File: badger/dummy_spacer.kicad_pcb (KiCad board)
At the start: 2 copper layers, 200 x 200 mm, 12 parts

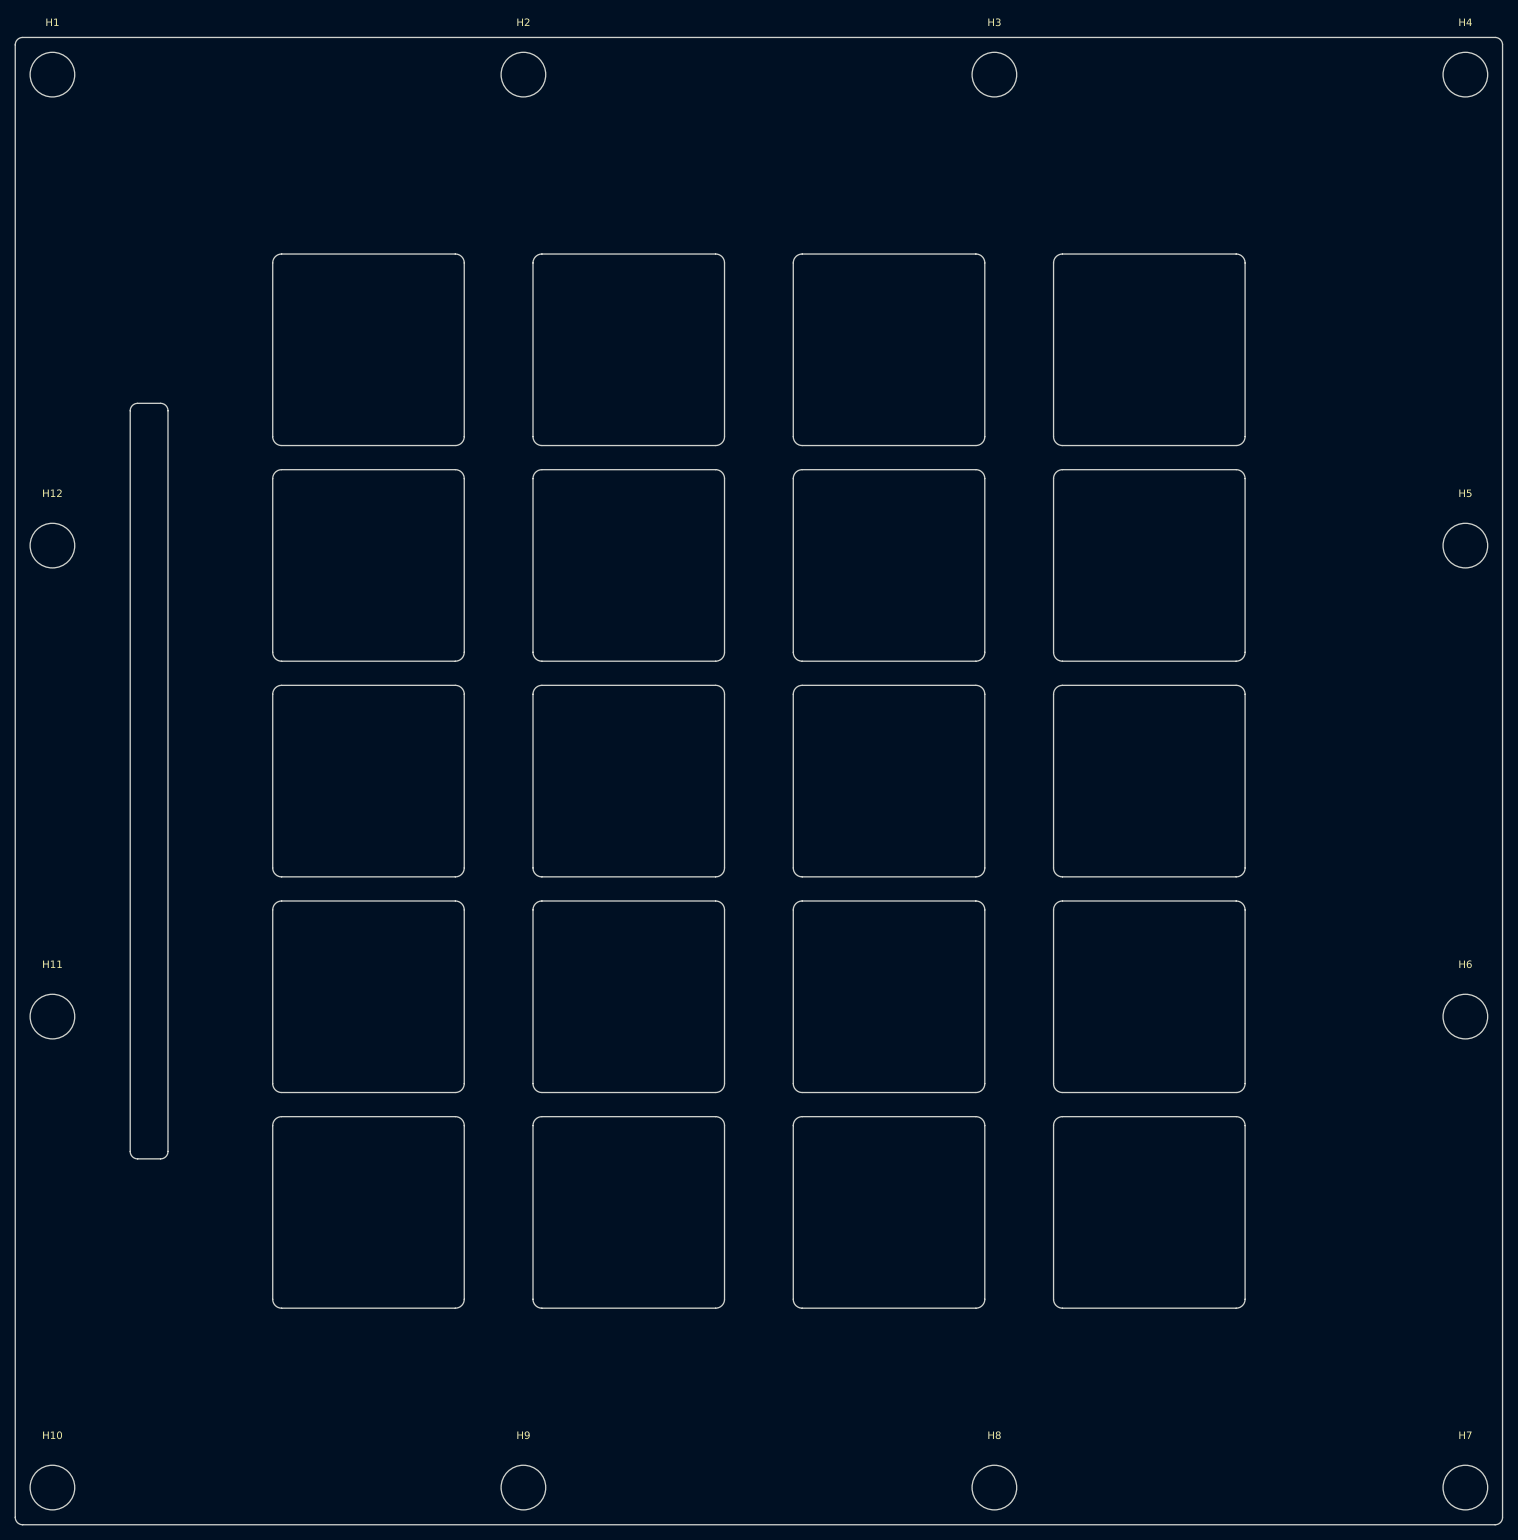
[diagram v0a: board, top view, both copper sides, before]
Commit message: badger upgrades
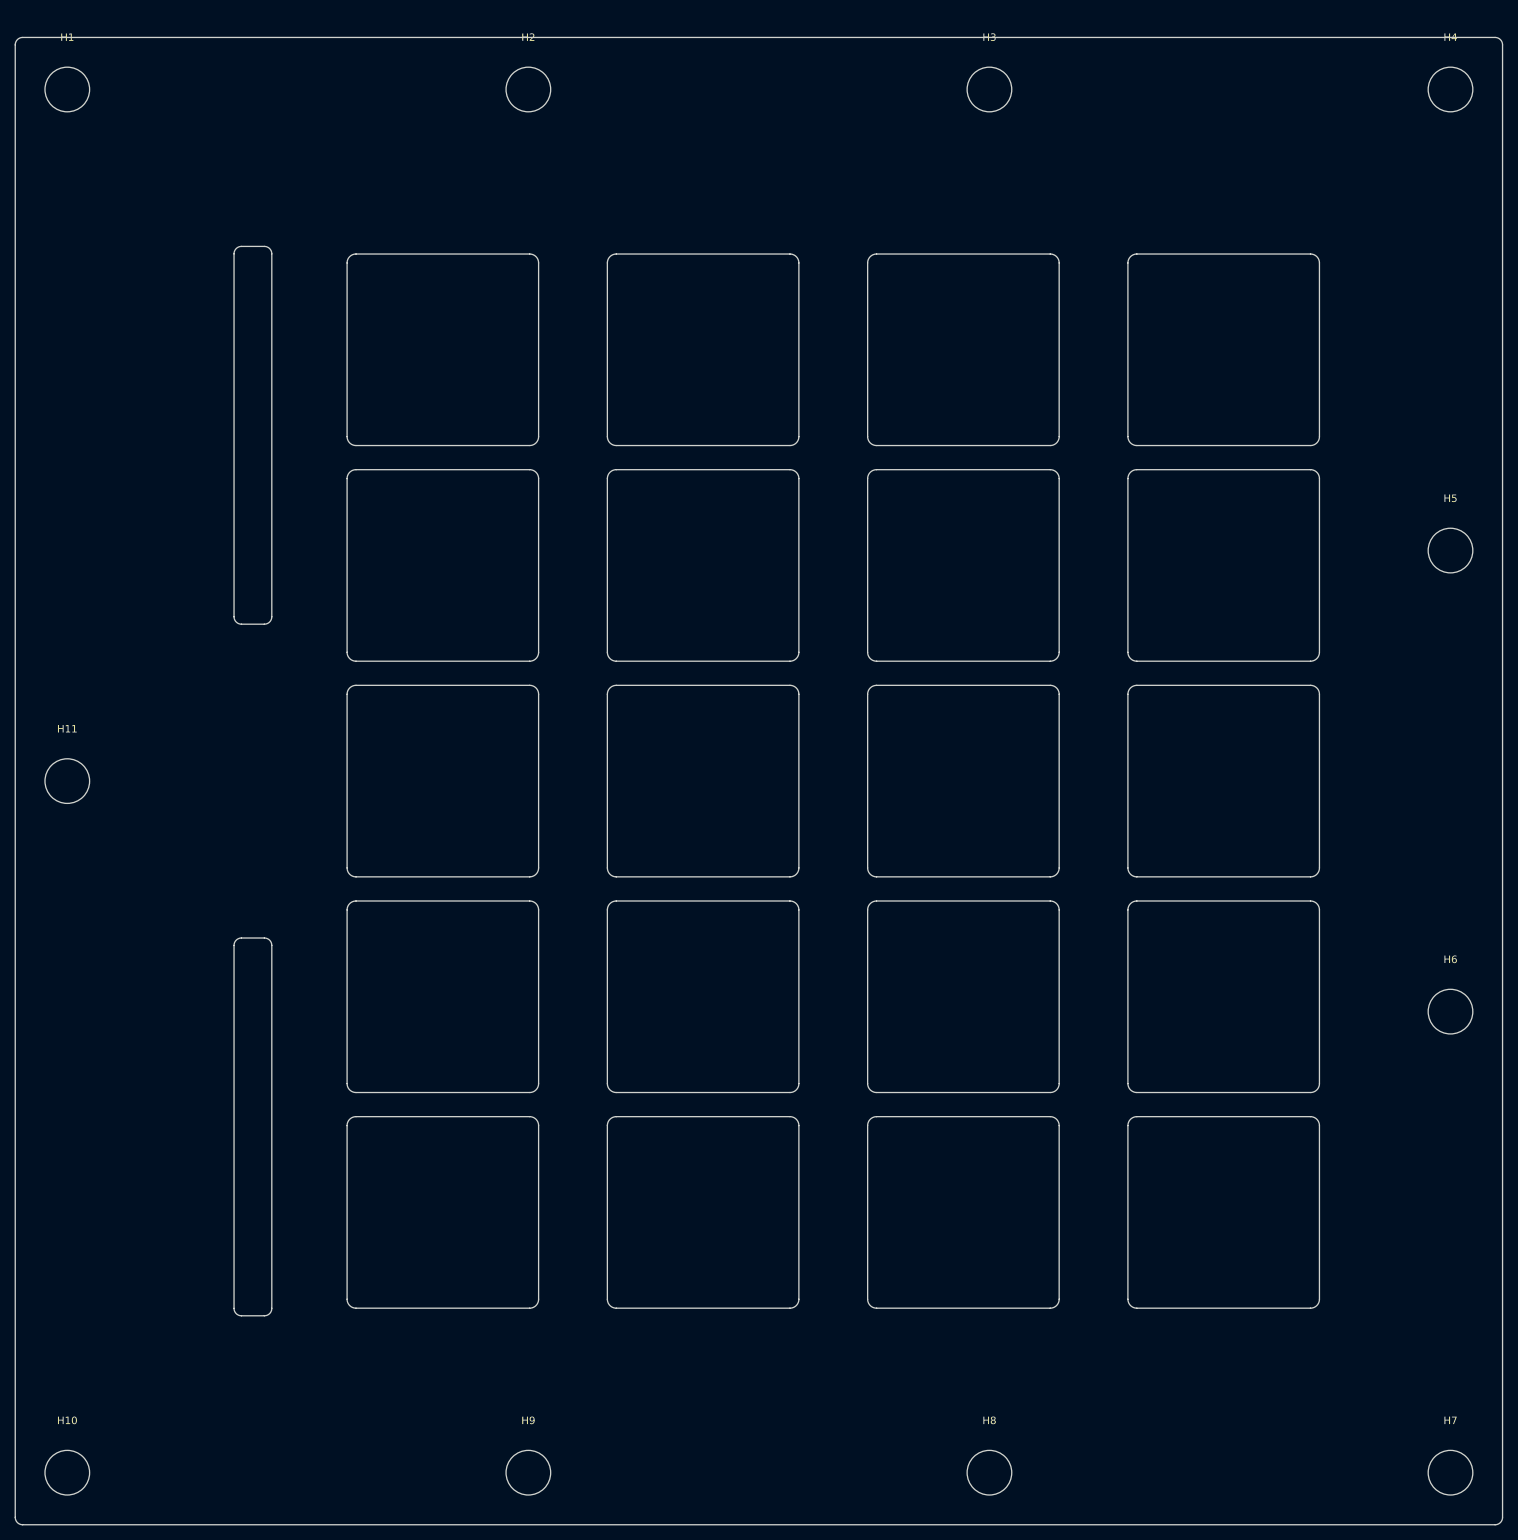
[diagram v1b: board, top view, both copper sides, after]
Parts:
- removed H12: MountingHole, MountingHole:MountingHole_6mm
- moved H11 31.7 mm to (-93.0, 0.00)
- moved H1 2.83 mm to (-93.0, -93.0)
- moved H10 2.83 mm to (-93.0, 93.0)
- moved H4 2.83 mm to (93.0, -93.0)
- moved H7 2.83 mm to (93.0, 93.0)
- moved H2 2.11 mm to (-31.0, -93.0)
- moved H3 2.11 mm to (31.0, -93.0)
- moved H5 2.11 mm to (93.0, -31.0)
- moved H6 2.11 mm to (93.0, 31.0)
- moved H8 2.11 mm to (31.0, 93.0)
- moved H9 2.11 mm to (-31.0, 93.0)
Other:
- outline, holes or cut-outs redrawn
